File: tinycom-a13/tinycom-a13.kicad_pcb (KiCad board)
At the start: 4 copper layers, 39.4 x 41.1 mm, 23 parts, among them P1 CONN_02X08, P2 CONN_02X08, U1 IC_A13, U2 H5TQ2G83BFR/FBGA82, Y1 Crystal

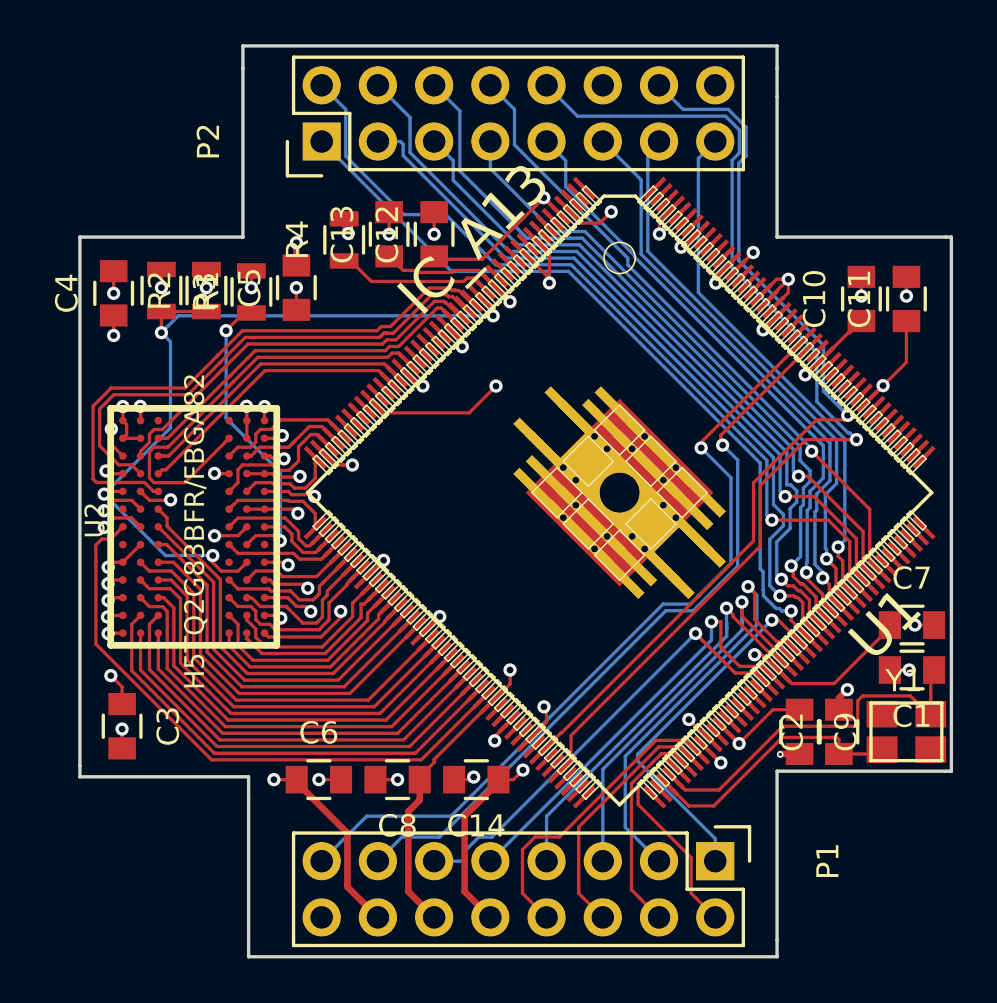
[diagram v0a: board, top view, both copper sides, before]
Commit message: prepare base
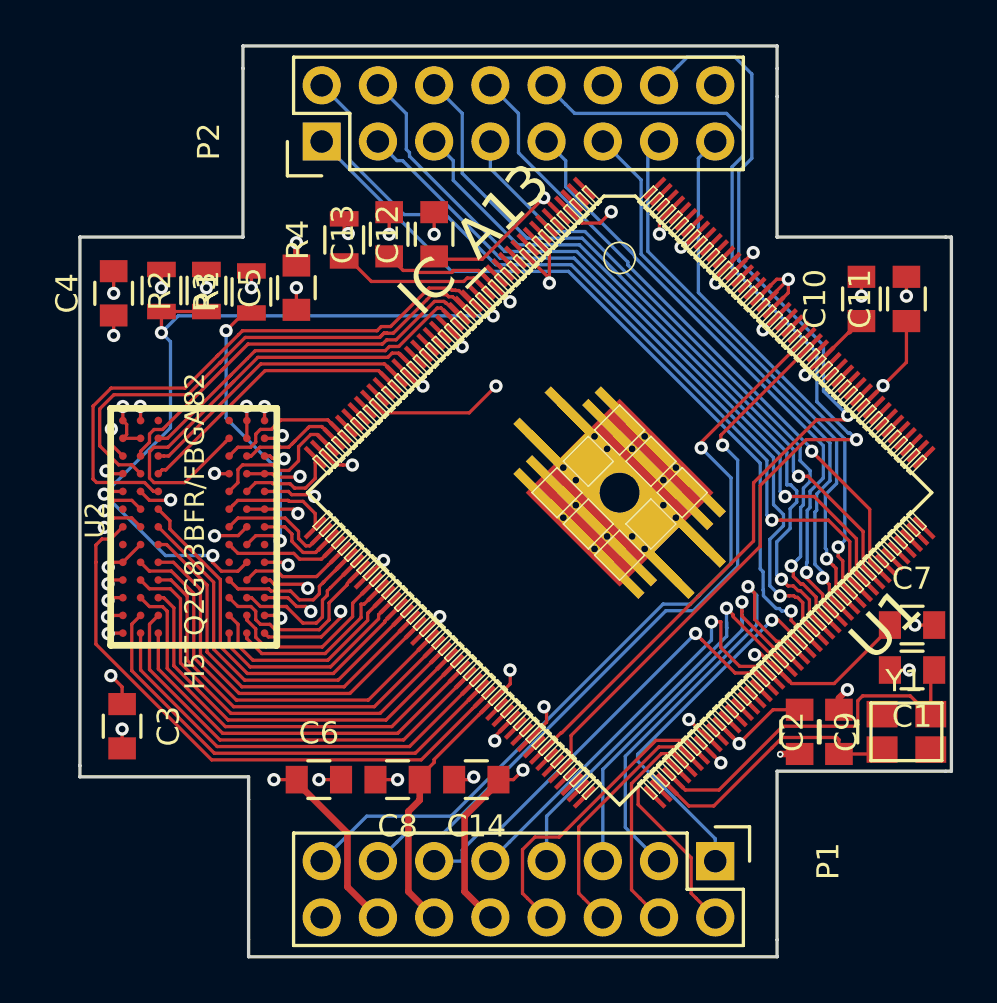
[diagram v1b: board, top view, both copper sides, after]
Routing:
- net VCC_30: track 42.4 -> 45.3 mm
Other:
- rule pad_to_mask_clearance: 0.2 -> 0.07
